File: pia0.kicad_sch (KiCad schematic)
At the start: 29 parts, among them IC20 MC14529B, IC24 74LS244N, IC25 LM393P, IC26 MC6821

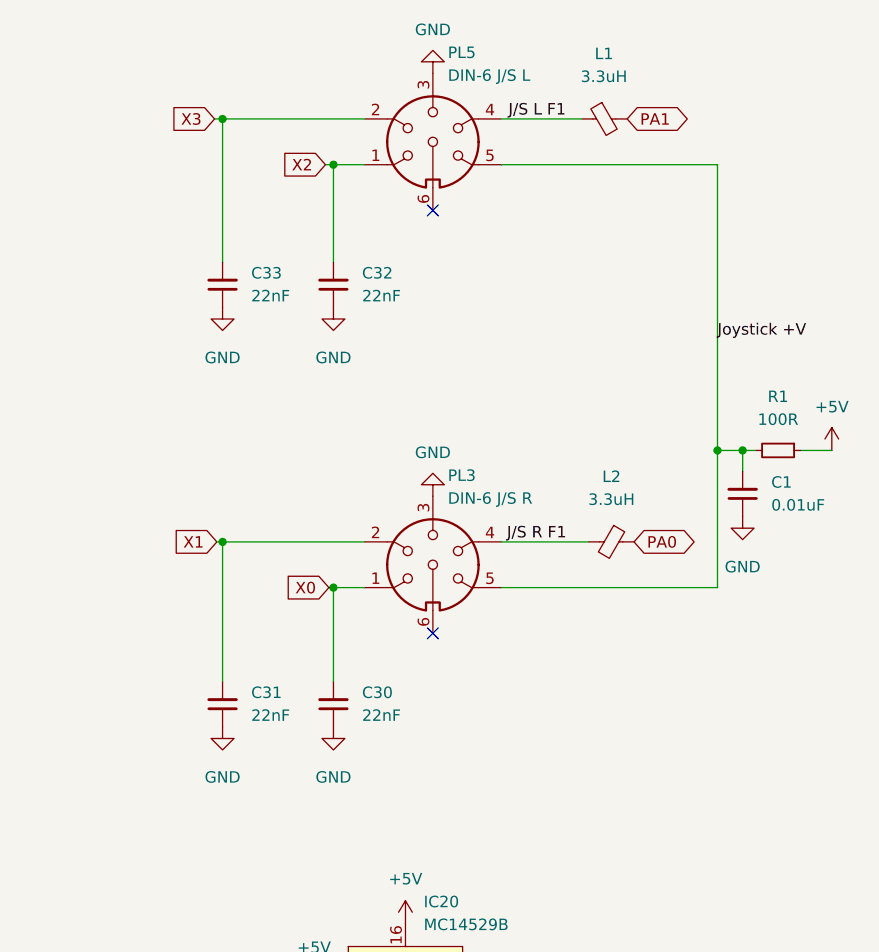
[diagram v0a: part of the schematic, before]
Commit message: video circuit tracing
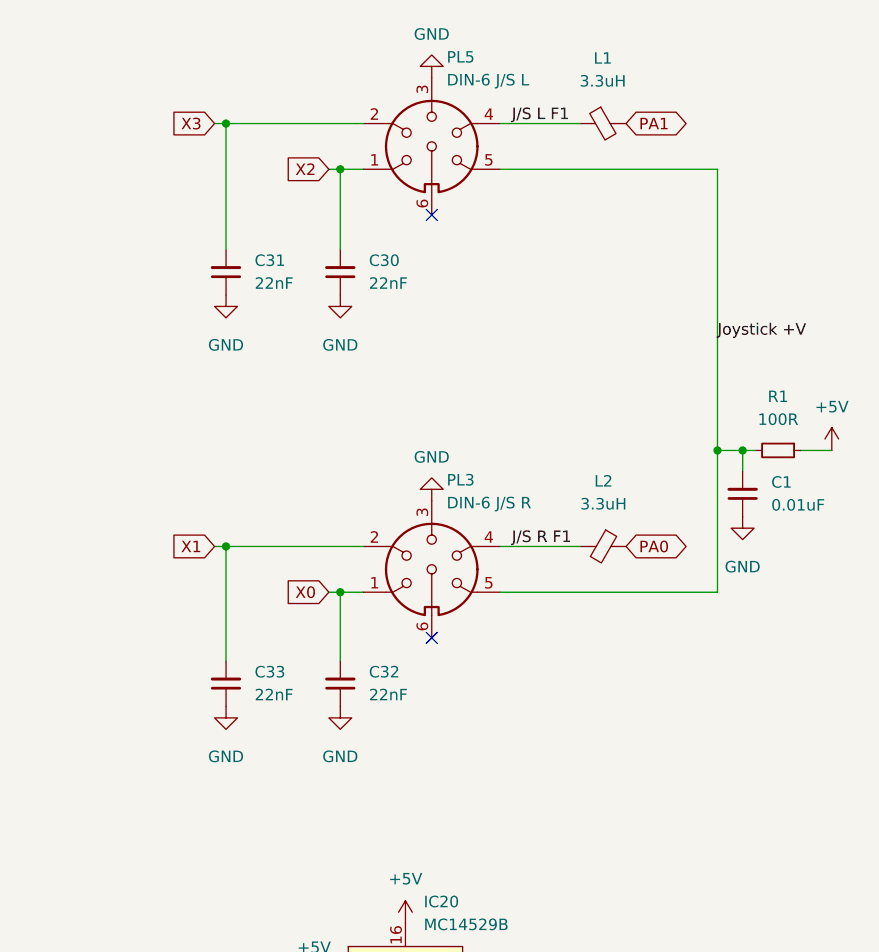
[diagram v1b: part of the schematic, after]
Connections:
- net X0: now also C32.2; no longer C30.2
- net X1: now also C33.2; no longer C31.2
- net X2: now also C30.2; no longer C32.2
- net X3: now also C31.2; no longer C33.2
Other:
- moved on the sheet: C30, C31, C32, C33, L1, L2, PL3, PL5
